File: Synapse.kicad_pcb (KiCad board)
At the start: 2 copper layers, 50 x 50 mm, 48 parts, among them J1 Conn_01x04_Female, Q1 Q_PMOS_GSD, -3.6A 0.02R, Q2 Q_NMOS_GSD 1Amp, SW1 SW_SPST, SW2 SW_SPST, U1 STM32F411CEUx, U2 SOT-23-3 LDO, U3 24LC256, Y1 25MHz 9pF, Y2 32.768K 7p

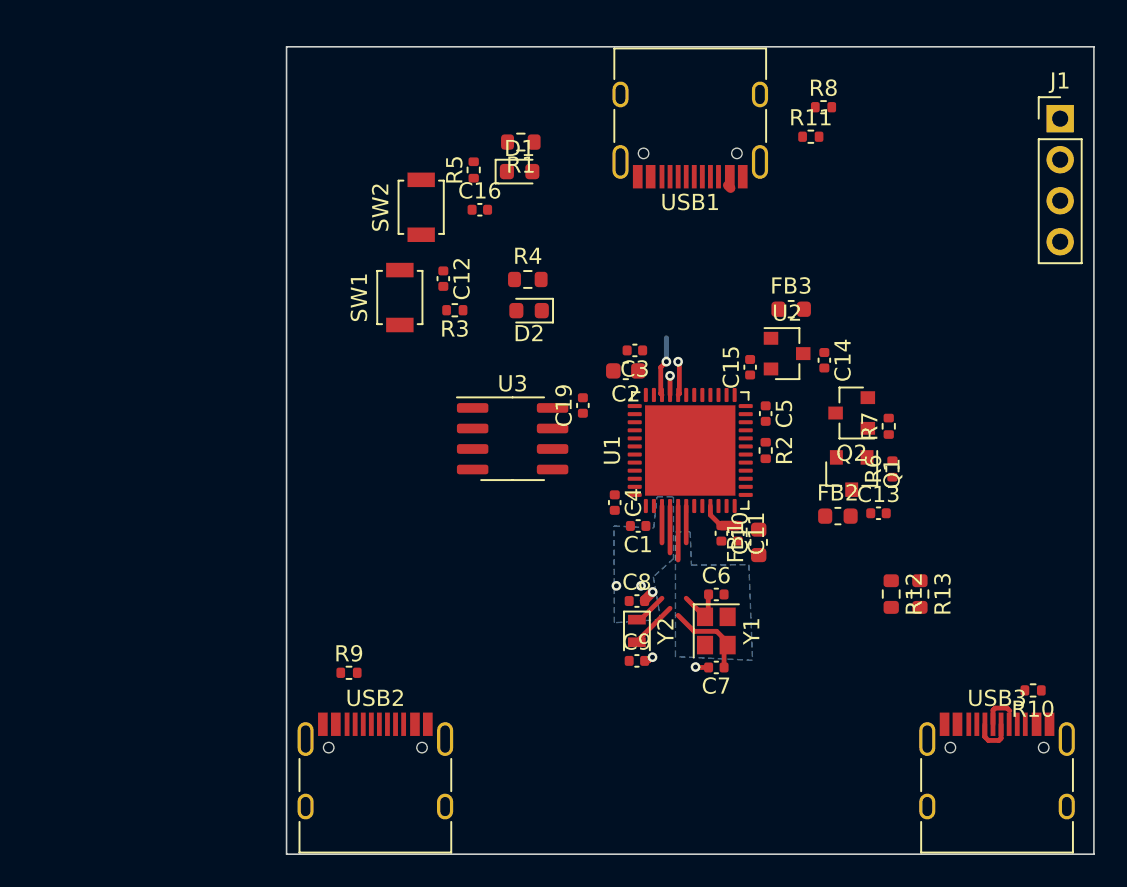
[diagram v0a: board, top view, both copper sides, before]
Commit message: PAUSED: Use `git resume` to continue working.
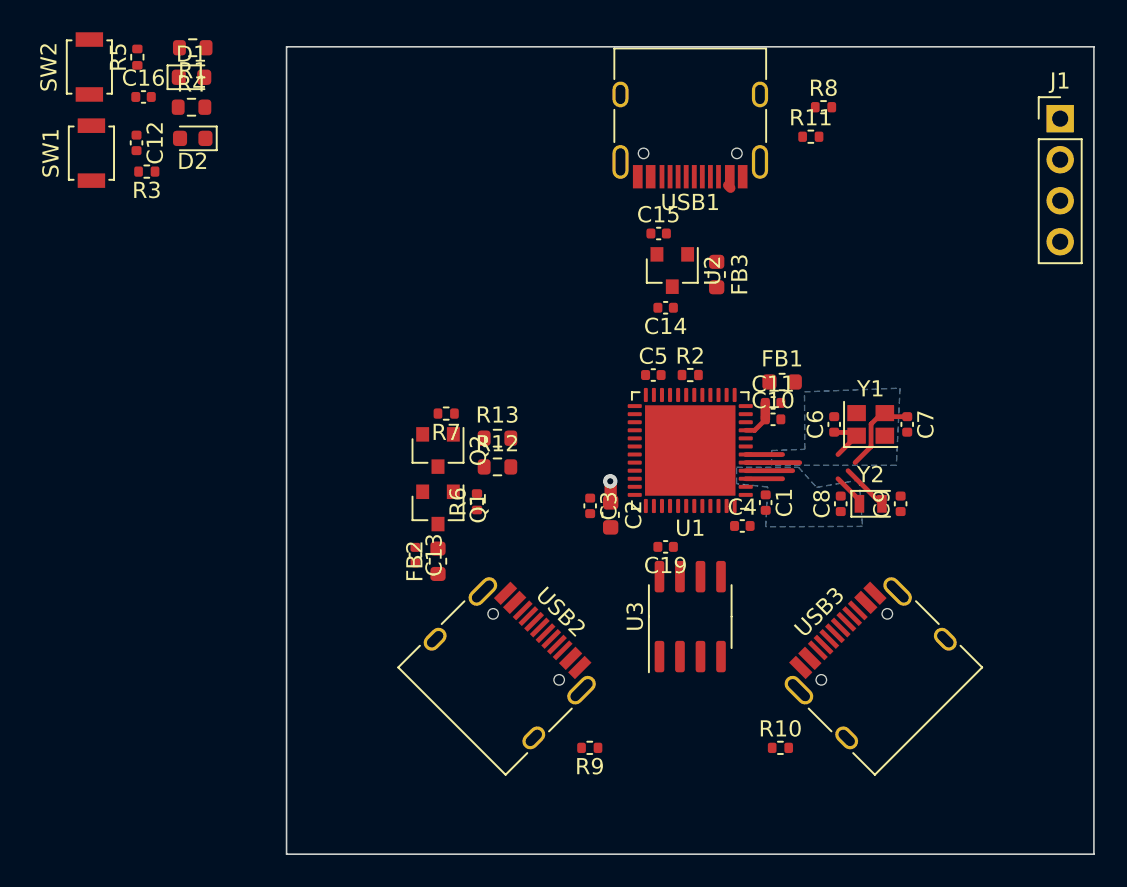
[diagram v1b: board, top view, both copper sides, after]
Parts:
- moved C13 28.8 mm to (-17.0, 6.48), turned to 270 degrees
- moved R13 27.9 mm to (-11.9, -0.76), turned to 0 degrees
- moved R7 27.4 mm to (-15.1, -2.29), turned to 180 degrees
- moved R6 25.8 mm to (-13.2, 3.17)
- moved Q2 25.7 mm to (-15.6, 0.00), turned to 270 degrees
- moved Q1 25.7 mm to (-15.6, 3.56)
- moved R12 25.6 mm to (-11.9, 1.02), turned to 0 degrees
- moved FB2 24.9 mm to (-15.6, 6.86), turned to 90 degrees
- moved D2 23.4 mm to (-30.8, -19.3)
- moved R4 23.4 mm to (-30.9, -21.3)
- moved SW2 22.3 mm to (-37.2, -23.7)
- moved C16 22.0 mm to (-33.9, -21.9)
- moved R5 22.0 mm to (-34.2, -24.4)
- moved D1 21.1 mm to (-30.9, -23.1)
- moved R1 21.1 mm to (-30.8, -24.9)
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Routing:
- net SWDIO: track 3.72 -> 0.00 mm, vias 1 -> 0
- net I2C1_SDA: track 2.80 -> 0.00 mm
- net GND: track 2.16 -> 0.00 mm, vias 5 -> 0
- net DN: track 2.13 -> 0.00 mm, vias 1 -> 0
- net I2C1_SCL: track 2.03 -> 0.00 mm
- net +3V3: track 0.00 -> 1.32 mm, vias 0 -> 1
- net DP: track 1.19 -> 0.00 mm, vias 1 -> 0
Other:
- copper layers 2 -> 4
- net class Default: trace_width 0.127 -> 0.254
- net class GND removed
- rule trace_min: 0.127 -> 0.09
- rule via_min_drill: 0.3 -> 0.2
- rule via_min_size: 0.6 -> 0.4
